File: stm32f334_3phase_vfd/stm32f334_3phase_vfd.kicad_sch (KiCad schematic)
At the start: 0 parts

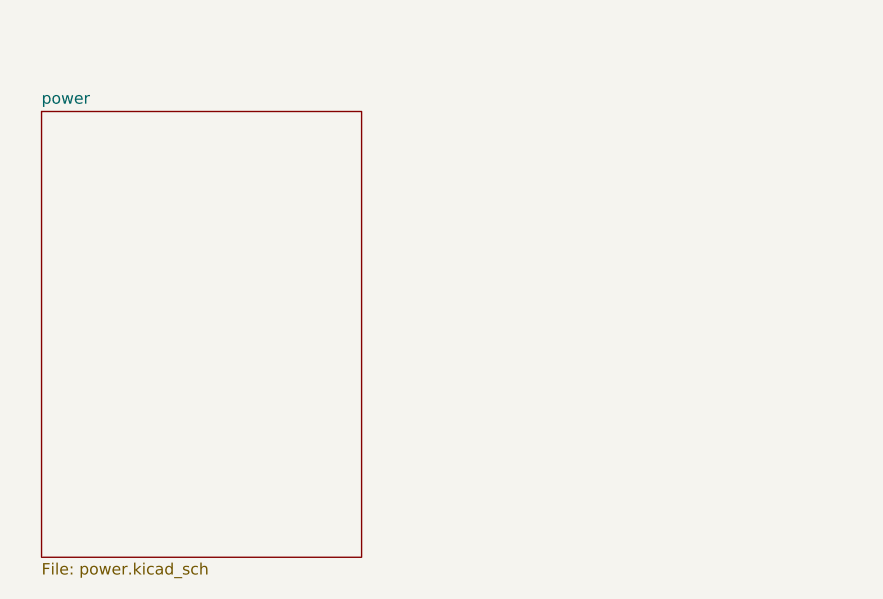
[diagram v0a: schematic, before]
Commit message: continue schematic work
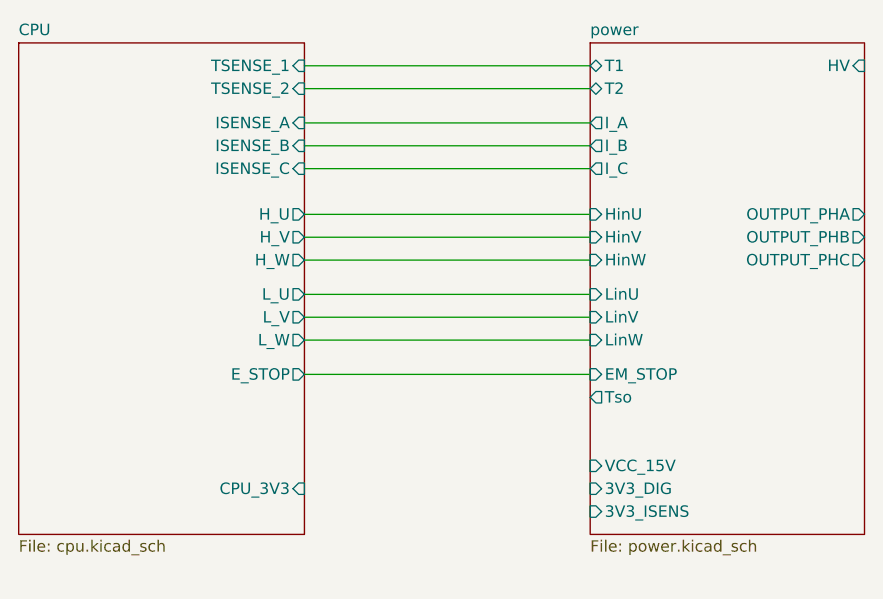
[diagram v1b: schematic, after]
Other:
- added sheet CPU (cpu.kicad_sch)
- sheet power ports: added 3V3_DIG, 3V3_ISENS, EM_STOP, HV, HinU, HinV, HinW, I_A, I_B, I_C, LinU, LinV, LinW, OUTPUT_PHA, OUTPUT_PHB, OUTPUT_PHC, T1, T2, Tso, VCC_15V; removed none
